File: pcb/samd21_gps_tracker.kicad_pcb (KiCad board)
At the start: 4 copper layers, 99 x 38.5 mm, 95 parts, among them J1 JTAG_SWD_6, J2 01x04, J3 U.FL-R-SMT, J4 SIM_Card, J5 USB_C_Receptacle_USB2.0, J6 U.FL-R-SMT, J7 C7244, Q1 2N7002, Q2 2N7002, Q3 2N7002, Q4 2N7002, Q5 2N7002, Q6 Q_PMOS_GSD, Q7 Q_PMOS_GSD, Q8 Q_PMOS_GSD, Q9 2N7002, SW1 SW_Push, SW2 SW_Push_SPDT, U1 XL1509_SOP8, U2 ATSAMD21G18A-A, U3 MCP2515-xSO, U4 L96-M33, U5 RN2903, U6 MCP2551-I-SN, U7 LIS2DE12, U8 SIM7020E, U9 ME6208, Y1 32.768k, Y2 16mHz

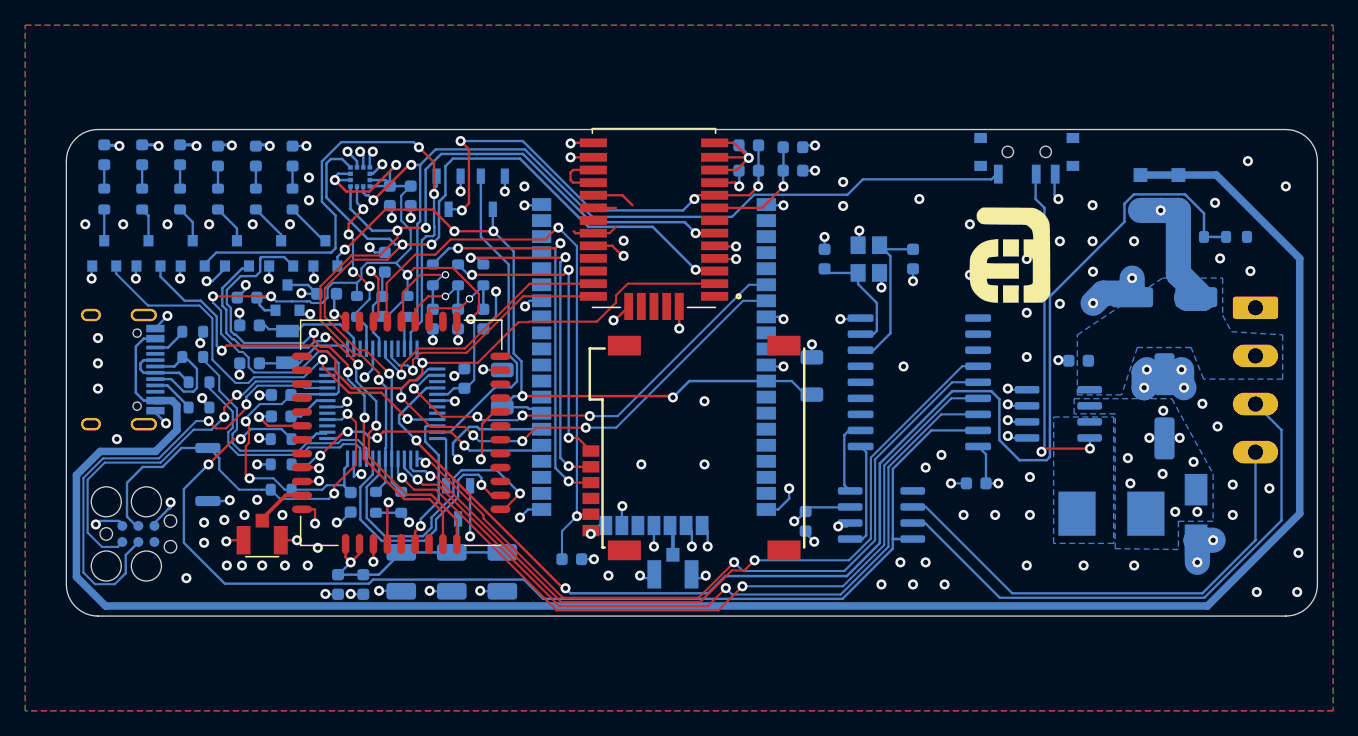
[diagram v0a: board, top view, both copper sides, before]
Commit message: WIP
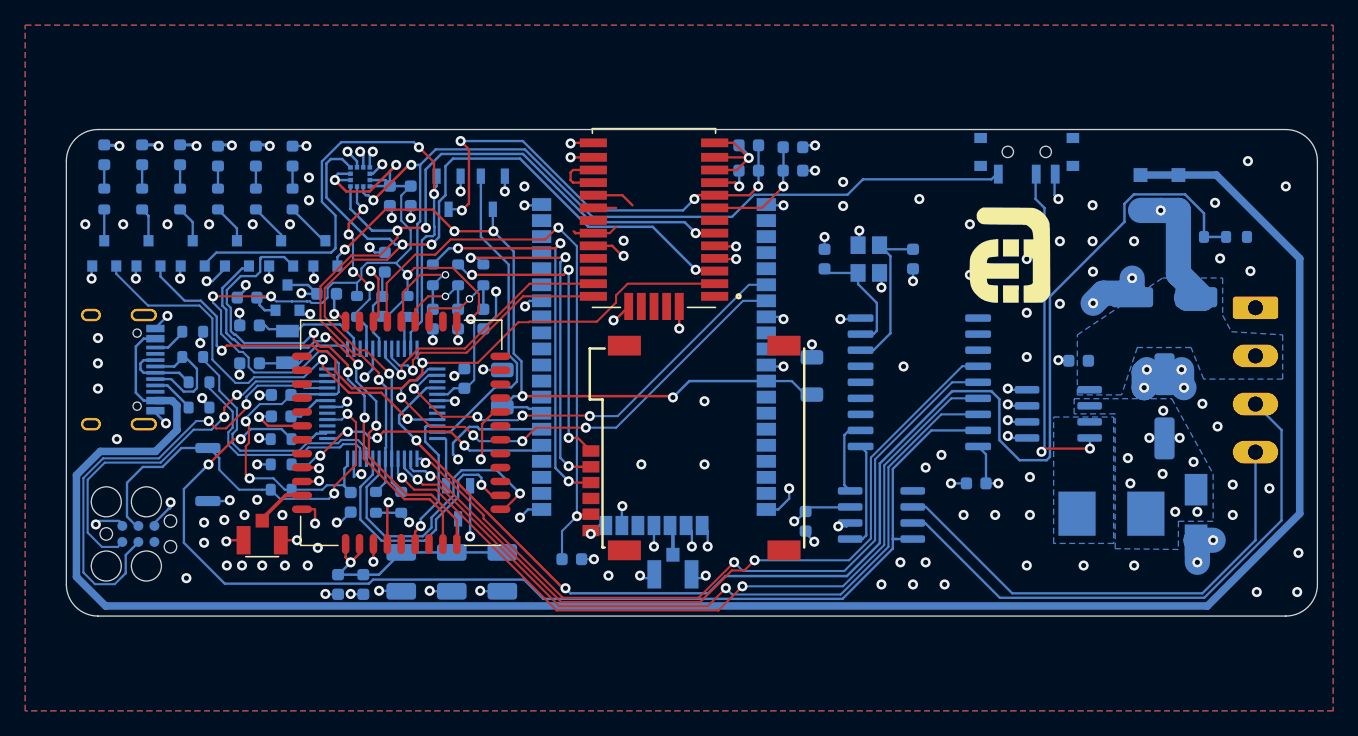
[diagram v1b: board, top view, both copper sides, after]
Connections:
- net ~EN renamed ~{EN}
- net ~Reset renamed ~{Reset}
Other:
- net class Default removed
